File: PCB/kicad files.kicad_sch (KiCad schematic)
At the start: 35 parts, among them J2 Conn_01x04_Pin, SW1 SW_Push_45deg, SW10 RotaryEncoder_Switch, SW2 SW_Push_45deg, SW3 SW_Push_45deg, SW4 SW_Push_45deg, SW5 SW_Push_45deg, SW6 SW_Push_45deg, SW7 SW_Push_45deg, SW8 SW_Push_45deg, SW9 SW_Push_45deg, U2 MOUDLE-SEEEDUINO-XIAO

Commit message: placed LEDs
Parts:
- renumbered D11 to D10, D7 to D11, D10 to D12, D8 to D13, D9 to D14, D15 to D2, D14 to D4, D4 to D5, D13 to D6, D5 to D7, D12 to D8, D6 to D9
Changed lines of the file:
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@@
 		(dnp no)
 		(fields_autoplaced yes)
-		(property "Reference" "D6"
+		(property "Reference" "D9"
 			(at 240.03 31.6798 0)
 			(hide yes)
@@
 			(project "kicad files"
 				(path "/88ceca4b-52c7-47e0-8744-4f7df2c73c46"
-					(reference "D6")
+					(reference "D9")
 					(unit 1)
 				)
@@
 		(dnp no)
 		(fields_autoplaced yes)
-		(property "Reference" "D11"
+		(property "Reference" "D10"
 			(at 189.23 75.0002 0)
 			(hide yes)
@@
 			(project "kicad files"
 				(path "/88ceca4b-52c7-47e0-8744-4f7df2c73c46"
-					(reference "D11")
+					(reference "D10")
 					(unit 1)
 				)
@@
 		(dnp no)
 		(fields_autoplaced yes)
-		(property "Reference" "D8"
+		(property "Reference" "D13"
 			(at 278.13 31.6798 0)
 			(hide yes)
@@
 			(project "kicad files"
 				(path "/88ceca4b-52c7-47e0-8744-4f7df2c73c46"
-					(reference "D8")
+					(reference "D13")
 					(unit 1)
 				)
@@
 		(dnp no)
 		(fields_autoplaced yes)
-		(property "Reference" "D9"
+		(property "Reference" "D14"
 			(at 227.33 75.0002 0)
 			(hide yes)
@@
 			(project "kicad files"
 				(path "/88ceca4b-52c7-47e0-8744-4f7df2c73c46"
-					(reference "D9")
+					(reference "D14")
 					(unit 1)
 				)
@@
 		(dnp no)
 		(fields_autoplaced yes)
-		(property "Reference" "D10"
+		(property "Reference" "D12"
 			(at 208.28 75.0002 0)
 			(hide yes)
@@
 			(project "kicad files"
 				(path "/88ceca4b-52c7-47e0-8744-4f7df2c73c46"
-					(reference "D10")
+					(reference "D12")
 					(unit 1)
 				)
@@
 		(dnp no)
 		(fields_autoplaced yes)
-		(property "Reference" "D5"
+		(property "Reference" "D7"
 			(at 220.98 31.6798 0)
 			(hide yes)
@@
 			(project "kicad files"
 				(path "/88ceca4b-52c7-47e0-8744-4f7df2c73c46"
-					(reference "D5")
+					(reference "D7")
 					(unit 1)
 				)
@@
 		(dnp no)
 		(fields_autoplaced yes)
-		(property "Reference" "D12"
+		(property "Reference" "D8"
 			(at 170.18 75.0002 0)
 			(hide yes)
@@
 			(project "kicad files"
 				(path "/88ceca4b-52c7-47e0-8744-4f7df2c73c46"
-					(reference "D12")
+					(reference "D8")
 					(unit 1)
 				)
@@
 		(dnp no)
 		(fields_autoplaced yes)
-		(property "Reference" "D4"
+		(property "Reference" "D5"
 			(at 201.93 31.6798 0)
 			(hide yes)
@@
 			(project "kicad files"
 				(path "/88ceca4b-52c7-47e0-8744-4f7df2c73c46"
-					(reference "D4")
+					(reference "D5")
 					(unit 1)
 				)
@@
 		(dnp no)
 		(fields_autoplaced yes)
-		(property "Reference" "D14"
+		(property "Reference" "D4"
 			(at 132.08 75.0002 0)
 			(hide yes)
@@
 			(project "kicad files"
 				(path "/88ceca4b-52c7-47e0-8744-4f7df2c73c46"
-					(reference "D14")
+					(reference "D4")
 					(unit 1)
 				)
@@
 		(dnp no)
 		(fields_autoplaced yes)
-		(property "Reference" "D15"
+		(property "Reference" "D2"
 			(at 113.03 75.0002 0)
 			(hide yes)
@@
 			(project "kicad files"
 				(path "/88ceca4b-52c7-47e0-8744-4f7df2c73c46"
-					(reference "D15")
+					(reference "D2")
 					(unit 1)
 				)
@@
 		(dnp no)
 		(fields_autoplaced yes)
-		(property "Reference" "D7"
+		(property "Reference" "D11"
 			(at 259.08 31.6798 0)
 			(hide yes)
@@
 			(project "kicad files"
 				(path "/88ceca4b-52c7-47e0-8744-4f7df2c73c46"
-					(reference "D7")
+					(reference "D11")
 					(unit 1)
 				)
@@
 		(dnp no)
 		(fields_autoplaced yes)
-		(property "Reference" "D13"
+		(property "Reference" "D6"
 			(at 151.13 75.0002 0)
 			(hide yes)
@@
 			(project "kicad files"
 				(path "/88ceca4b-52c7-47e0-8744-4f7df2c73c46"
-					(reference "D13")
+					(reference "D6")
 					(unit 1)
 				)

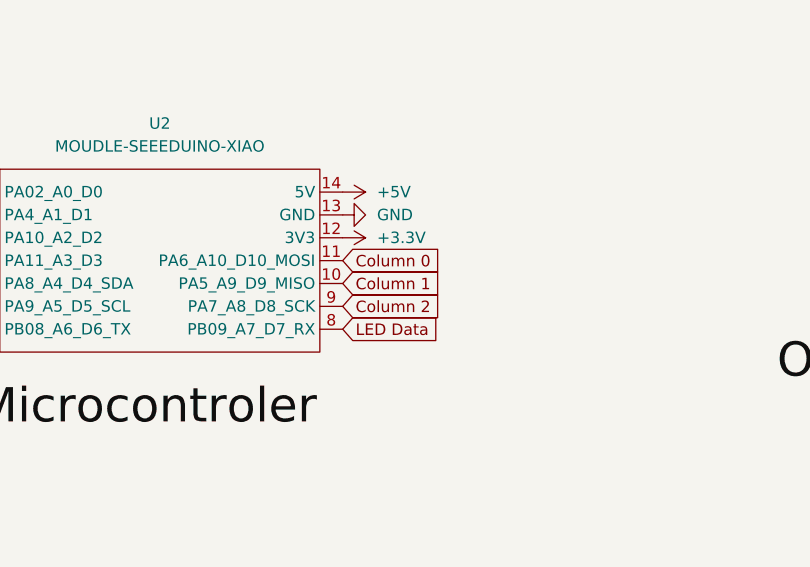
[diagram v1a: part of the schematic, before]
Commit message: pcb finally done with 64 fucking errorss
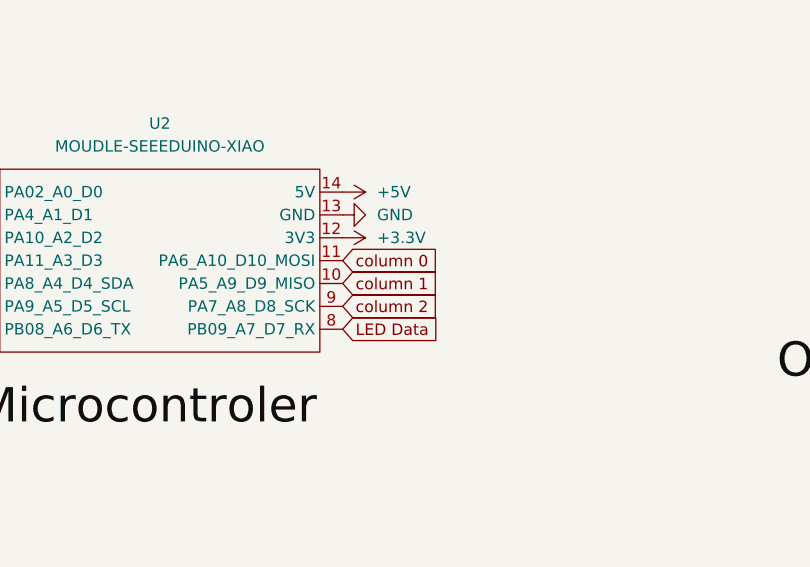
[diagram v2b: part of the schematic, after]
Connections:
- net Column 0 is gone; now on net column 0: U2.11 (PA6_A10_D10_MOSI)
- net Column 1 is gone; now on net column 1: U2.10 (PA5_A9_D9_MISO)
- net Column 2 is gone; now on net column 2: U2.9 (PA7_A8_D8_SCK)
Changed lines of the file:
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@@
 		)
 	)
-	(global_label "Column 1"
+	(global_label "column 1"
 		(shape input)
 		(at 163.83 127 0)
@@
 		)
 		(property "Intersheetrefs" "${INTERSHEET_REFS}"
-			(at 176.0678 127 0)
-			(hide yes)
-			(show_name no)
-			(do_not_autoplace no)
-			(effects
-				(font
-					(size 1.27 1.27)
-				)
-				(justify left)
-			)
-		)
-	)
-	(global_label "Column 0"
+			(at 175.8864 127 0)
+			(hide yes)
+			(show_name no)
+			(do_not_autoplace no)
+			(effects
+				(font
+					(size 1.27 1.27)
+				)
+				(justify left)
+			)
+		)
+	)
+	(global_label "column 0"
 		(shape input)
 		(at 163.83 124.46 0)
@@
 		)
 		(property "Intersheetrefs" "${INTERSHEET_REFS}"
-			(at 176.0678 124.46 0)
+			(at 175.8864 124.46 0)
 			(hide yes)
 			(show_name no)
@@
 		)
 	)
-	(global_label "Column 2"
+	(global_label "column 2"
 		(shape input)
 		(at 163.83 129.54 0)
@@
 		)
 		(property "Intersheetrefs" "${INTERSHEET_REFS}"
-			(at 176.0678 129.54 0)
-			(hide yes)
-			(show_name no)
+			(at 175.8864 129.54 0)
+			(hide yes)
+			(show_name no)
